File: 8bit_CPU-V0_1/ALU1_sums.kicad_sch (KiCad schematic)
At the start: 17 parts, among them U14 74LS283, U15 74LS283, U17 74LS32, U18 74LS08, U19 74HCT02, U20 74LS04, U21 74LS08, U6 74LS245, U8 74LS08

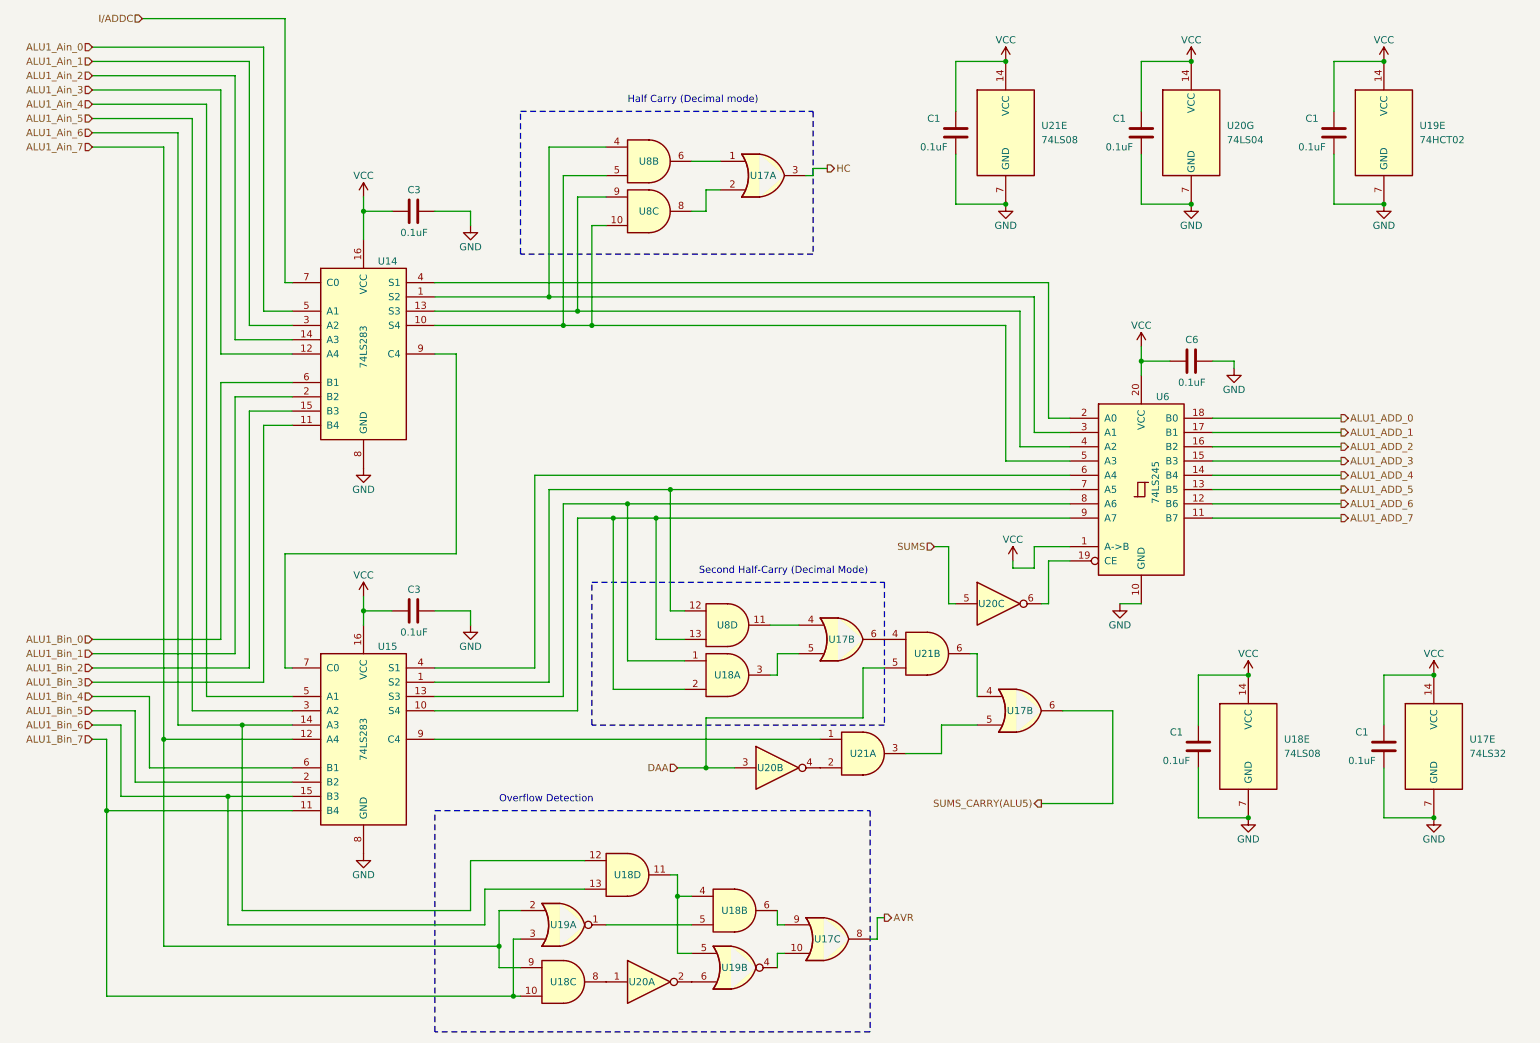
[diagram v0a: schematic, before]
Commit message: Refining schematics
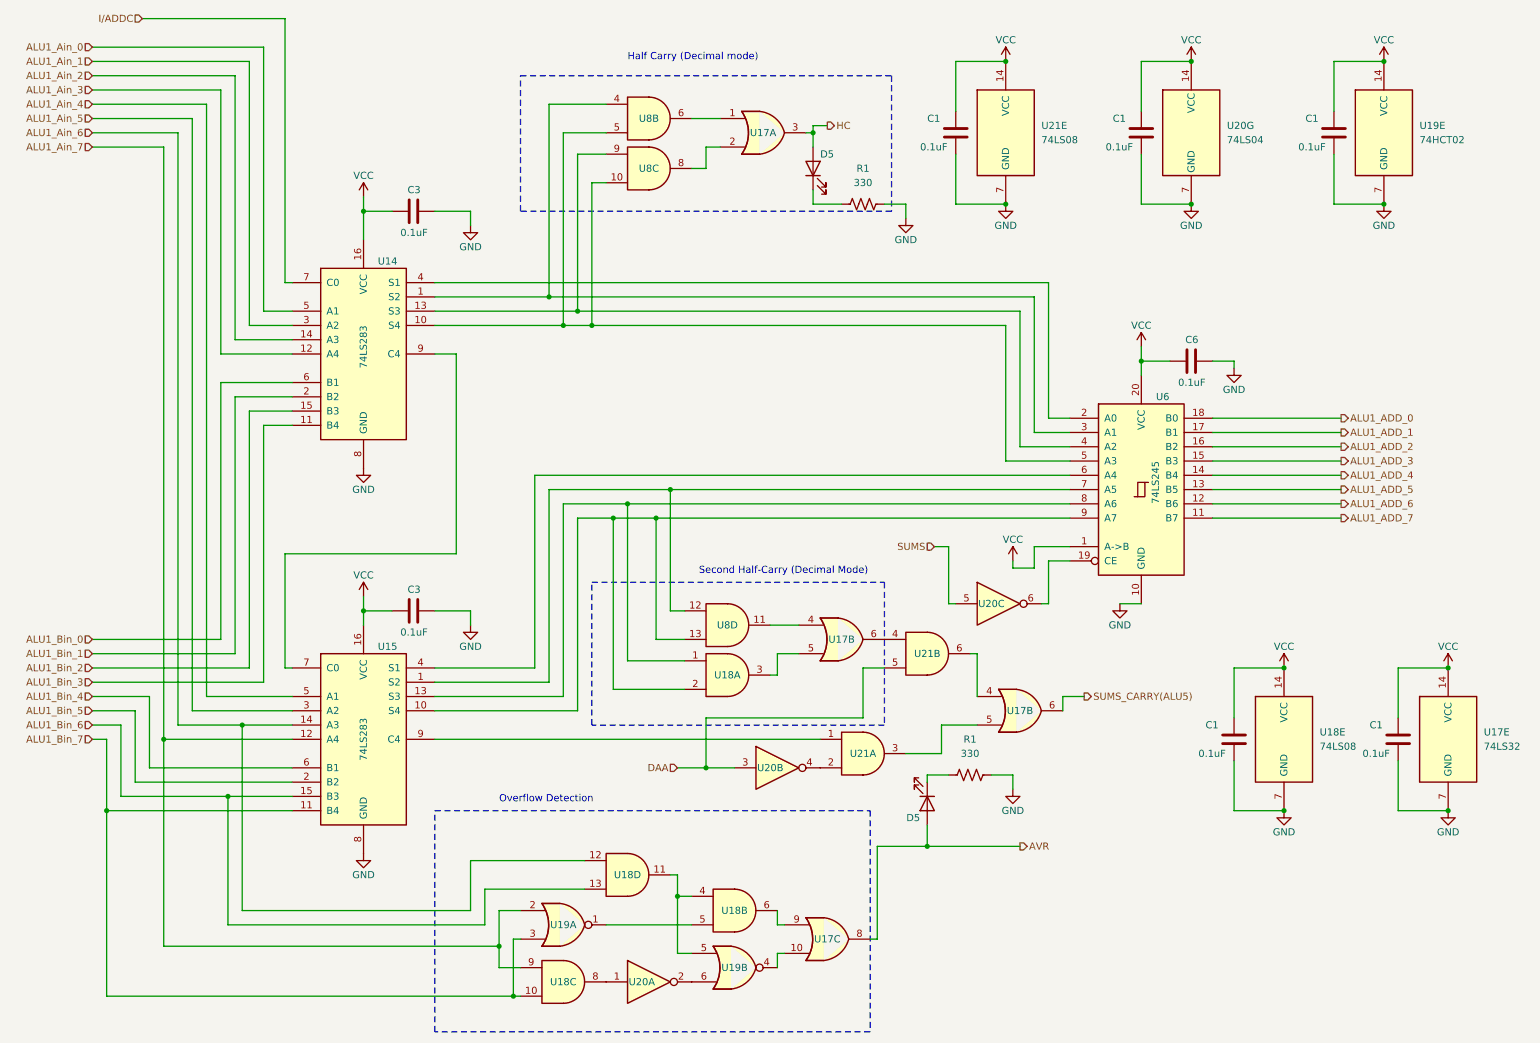
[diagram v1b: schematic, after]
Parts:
- added D5 (x2): LED, symbol Device:LED
- added R1 (x2): 330, symbol Device:R_US
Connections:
- net AVR: now also D5.2 (A)
- net GND: now also R1.2, R1.2
- net HC: now also D5.2 (A)
- new net: D5.1 (K), R1.1 (x2)
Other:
- moved on the sheet: C1, U17A, U17E, U18E, U8B, U8C

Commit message: New update
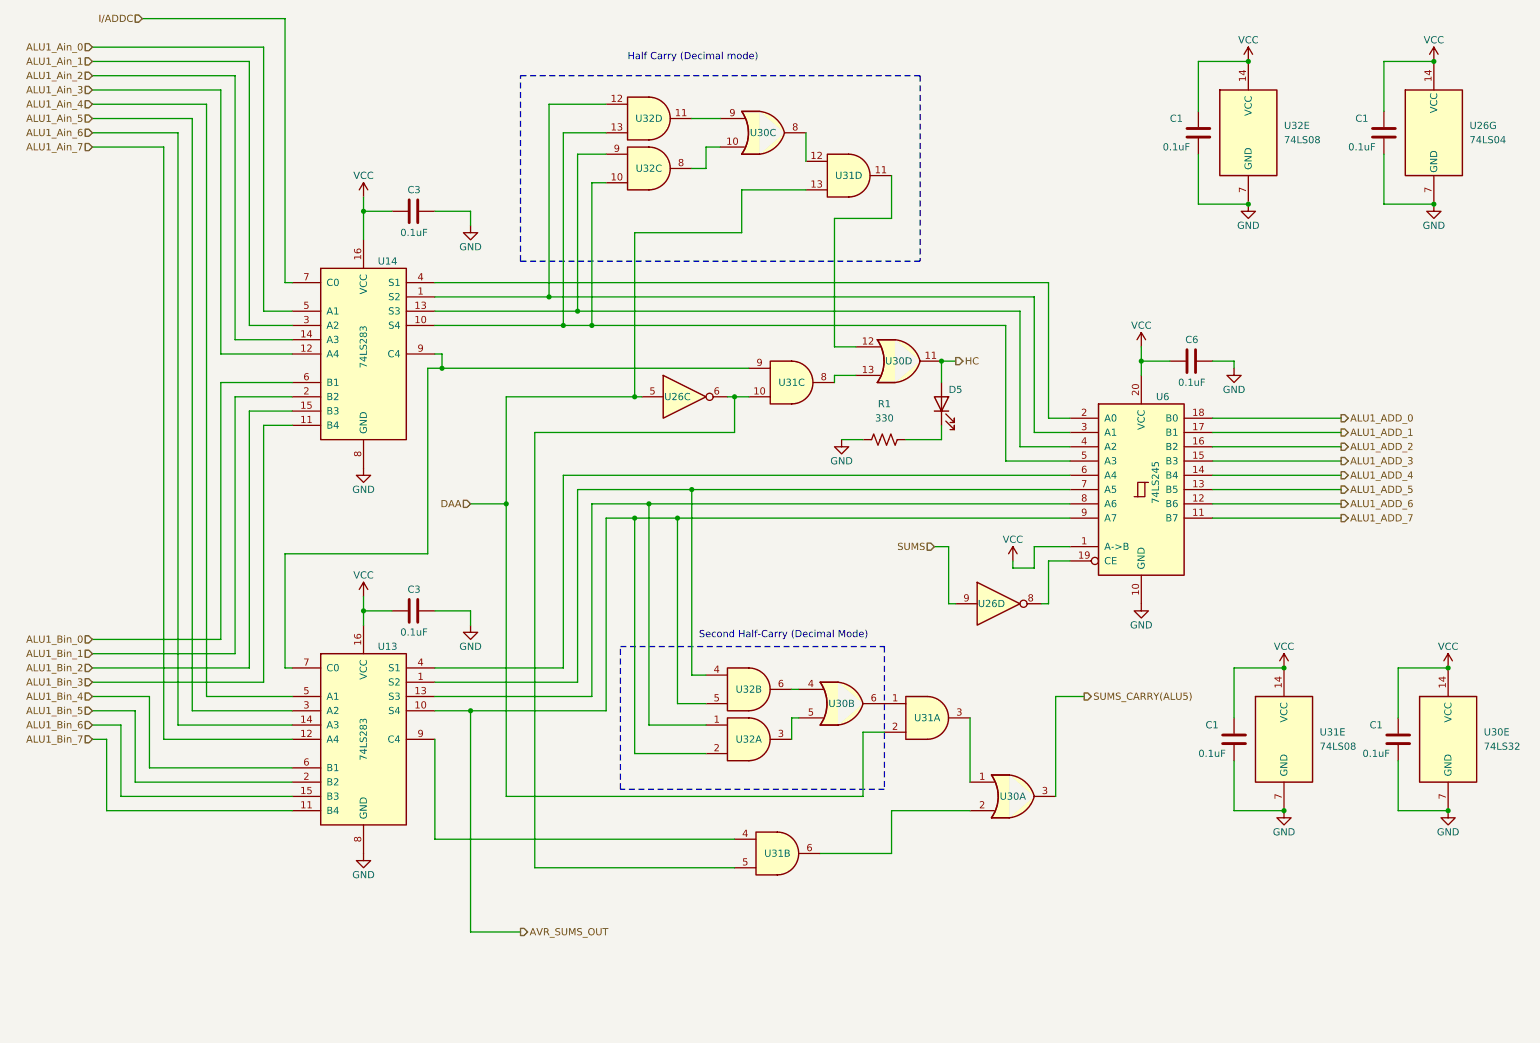
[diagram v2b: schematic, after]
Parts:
- removed C1: 0.1uF, symbol Device:C
- removed D5 (x2): LED, symbol Device:LED
- removed R1 (x2): 330, symbol Device:R_US
- removed unit 3 of U17
- removed unit 3 of U18
- removed unit 4 of U18
- removed unit 2 of U18
- removed U19: 74HCT02, symbol 74xx:74HCT02
- removed unit 2 of U20
- removed unit 1 of U20
- added D5: LED, symbol Device:LED
- added R1: 330, symbol Device:R_US
- added unit 3 of U26
- added unit 4 of U30
- added unit 3 of U31
- added unit 4 of U31
- renumbered U15 to U13, U20 to U26, U17 to U30, U21 to U31, U18 to U31, U8 to U32, U18 to U32, U21 to U32
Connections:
- net DAA: now also U31.2, U26.5, U31.13; no longer U31.5
- net GND: now also R1.1
- net HC: now also D5.2 (A), U30.11; no longer U30.3
- net SUMS: now also U26.9; no longer U26.5
- net SUMS_CARRY(ALU5): now also U30.3; no longer U30.6
- net at U14.10 (S4), U32.10, U6.5 (A3): now also U32.13; no longer U32.5
- net at U32.8: now also U30.10; no longer U30.2
- net at U30.4: now also U32.6; no longer U32.11
- net at U30.6: now also U31.1; no longer U31.4
- net AVR_SUMS_OUT: now reaches U13.10 (S4), U32.2, U6.9 (A7)
- net AVR_SUMS_OUT: now also U32.5; no longer U32.13
- net at U13.1 (S2), U6.7 (A5): now also U32.4; no longer U32.12
- net at U6.19 (CE): now also U26.8; no longer U26.6
- net at U14.1 (S2), U6.3 (A1): now also U32.12; no longer U32.4
- net at U13.9 (C4): now also U31.4; no longer U31.1
- net at U13.7 (C0), U14.9 (C4): now also U31.9
- new net: D5.1 (K), R1.2
- new net: U30.1, U31.3
- new net: U30.8, U31.12
- new net: U30.9, U32.11
- new net: U26.6, U31.10, U31.5
- new net: U30.2, U31.6
- new net: U30.13, U31.8
- new net: U30.12, U31.11
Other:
- note removed: "Overflow Detection"
- moved on the sheet: C1, U26G, U30A, U30B, U31A, U31B, U32A, U32B, U32E
